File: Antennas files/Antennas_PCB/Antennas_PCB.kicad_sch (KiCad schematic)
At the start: 13 parts, among them U1 LMR14030SDDA, U2 TSR_1-2433

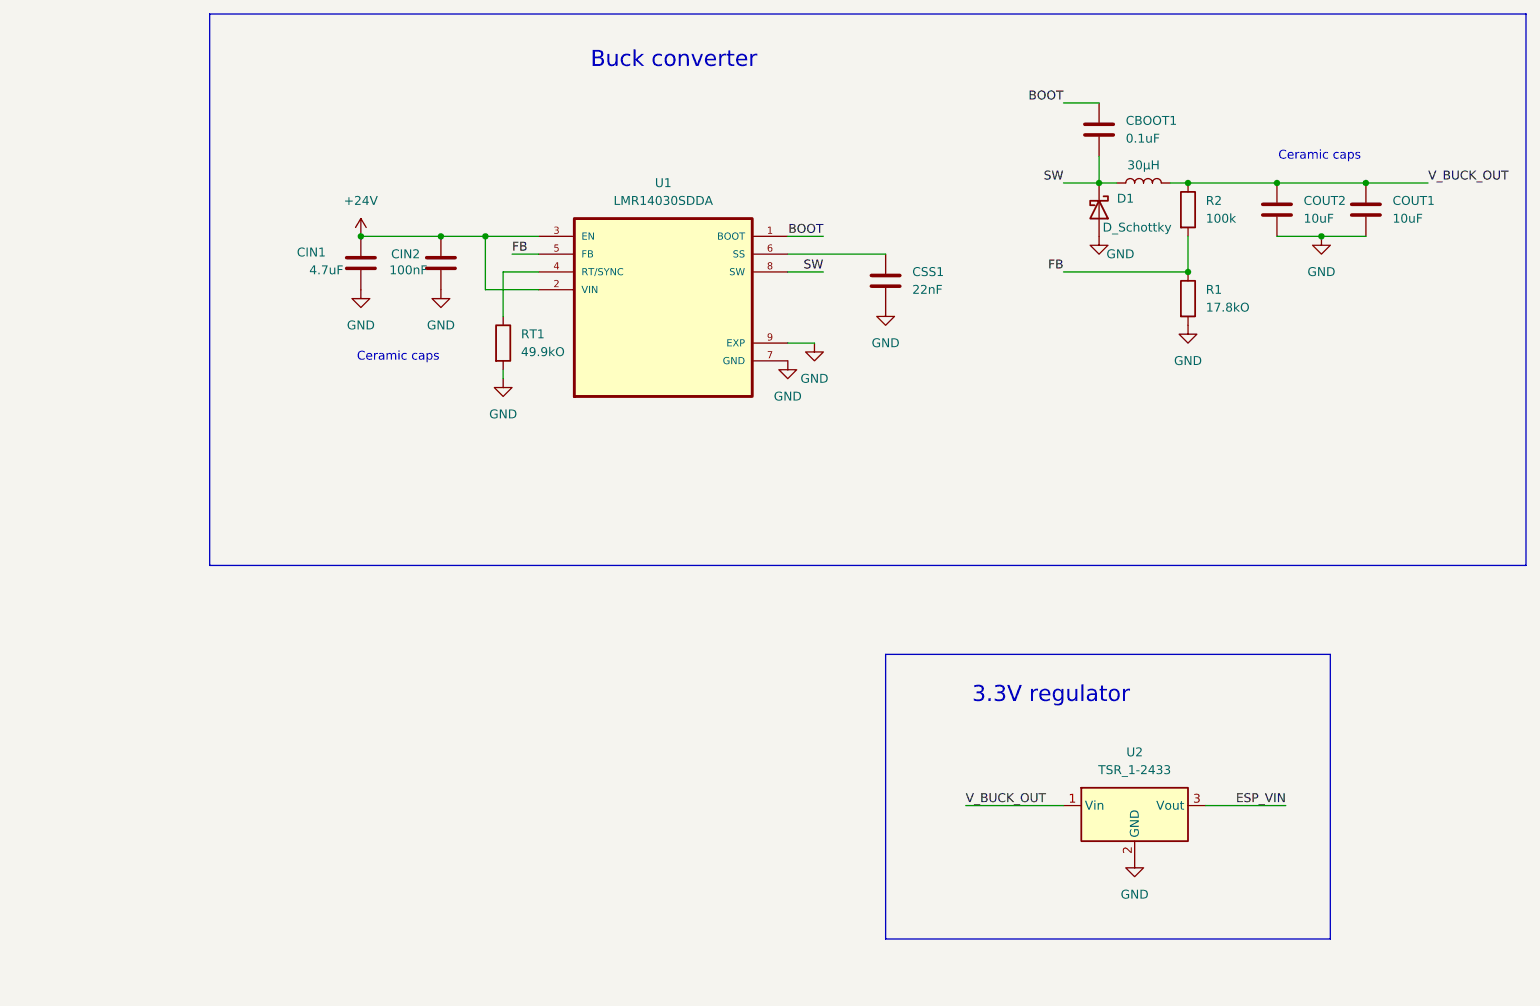
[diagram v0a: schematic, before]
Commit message: Add files via upload
pcb design for new buck and volt reg
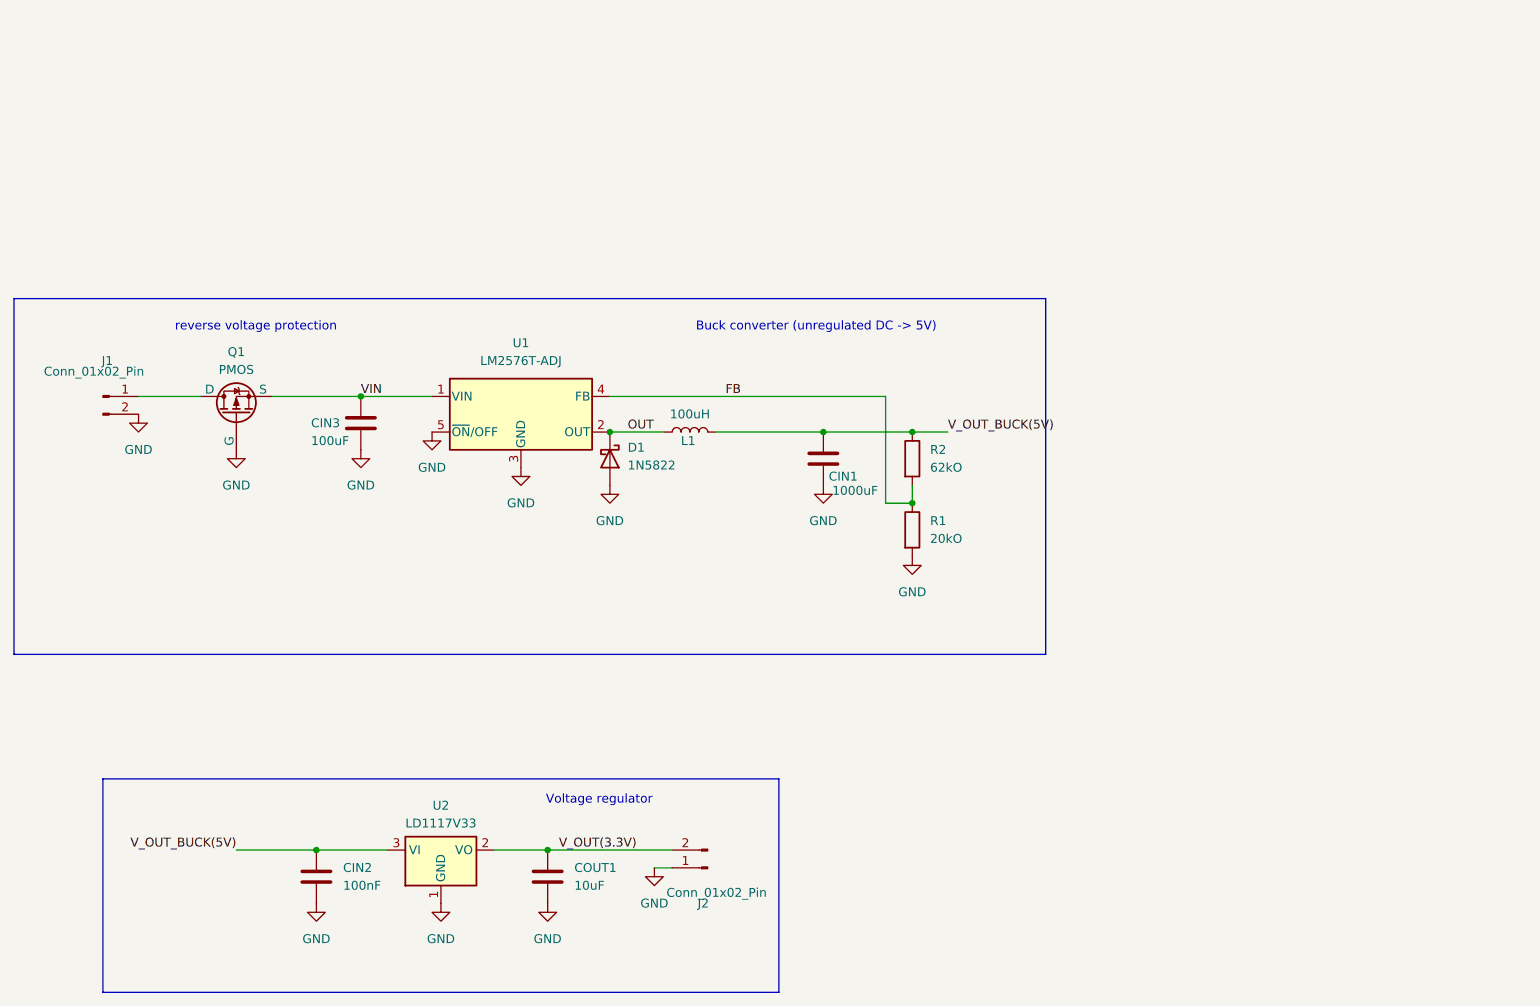
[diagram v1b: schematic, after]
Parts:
- removed CBOOT1: 0.1uF, Capacitor_SMD:C_0805_2012Metric_Pad1.18x1.45mm_HandSolder, symbol Device:C
- removed COUT2: 10uF, Capacitor_SMD:C_1206_3216Metric_Pad1.33x1.80mm_HandSolder, symbol Device:C
- removed CSS1: 22nF, Capacitor_SMD:C_0805_2012Metric_Pad1.18x1.45mm_HandSolder, symbol Device:C
- removed RT1: 49.9kO, Resistor_SMD:R_0805_2012Metric_Pad1.20x1.40mm_HandSolder, symbol Device:R
- removed U1: LMR14030SDDA, Package_SO:Texas_R-PDSO-G8_EP2.95x4.9mm_Mask2.4x3.1mm, symbol LMR14030SDDA:LMR14030SDDA
- removed U2: TSR_1-2433, Converter_DCDC:Converter_DCDC_TRACO_TSR-1_THT, symbol Converter_DCDC:TSR_1-2433
- added CIN3: 100uF, Capacitor_THT:C_Disc_D5.0mm_W2.5mm_P5.00mm, symbol Device:C
- added J1, J2: Conn_01x02_Pin, Connector_PinHeader_1.00mm:PinHeader_1x02_P1.00mm_Vertical, symbol Connector:Conn_01x02_Pin
- added Q1: PMOS, my_library:Untitled, symbol Simulation_SPICE:PMOS
- added U1: LM2576T-ADJ, Package_TO_SOT_THT:TO-220-5_Vertical, symbol Regulator_Switching:LM2576T-ADJ
- added U2: LD1117V33, Package_TO_SOT_THT:TO-220-3_Vertical, symbol Regulator_Linear:LD1117V33
- CIN1: value 4.7uF -> 1000uF; footprint Capacitor_SMD:C_0805_2012Metric_Pad1.18x1.45mm_HandSolder -> Capacitor_THT:C_Disc_D5.0mm_W2.5mm_P5.00mm
- CIN2: footprint Capacitor_SMD:C_0805_2012Metric_Pad1.18x1.45mm_HandSolder -> Capacitor_THT:C_Disc_D5.0mm_W2.5mm_P5.00mm
- COUT1: footprint Capacitor_SMD:C_1206_3216Metric_Pad1.33x1.80mm_HandSolder -> Capacitor_THT:C_Disc_D5.0mm_W2.5mm_P5.00mm
- D1: value D_Schottky -> 1N5822; footprint (none) -> Diode_THT:D_DO-201AD_P12.70mm_Horizontal
- L1: value 30µH -> 100uH; footprint (none) -> Inductor_THT:L_Axial_L6.6mm_D2.7mm_P10.16mm_Horizontal_Vishay_IM-2
- R1: value 17.8kO -> 20kO; footprint Resistor_SMD:R_0805_2012Metric_Pad1.20x1.40mm_HandSolder -> Resistor_THT:R_Axial_DIN0207_L6.3mm_D2.5mm_P10.16mm_Horizontal
- R2: value 100k -> 62kO; footprint Resistor_SMD:R_0805_2012Metric_Pad1.20x1.40mm_HandSolder -> Resistor_THT:R_Axial_DIN0207_L6.3mm_D2.5mm_P10.16mm_Horizontal
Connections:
- net FB: now also U1.4 (FB)
- net +24V renamed V_OUT_BUCK(5V)
- net V_OUT_BUCK(5V): now also L1.2, R2.1, U2.3 (VI)
- net EXP renamed GND
- net GND: now also CIN3.2, J1.2 (Pin_2), J2.1 (Pin_1), Q1.2 (G), U1.3 (GND), U1.5 (~{ON}/OFF), U2.1 (GND)
- net SW renamed OUT
- net OUT: now also U1.2 (OUT)
- removed net V_BUCK_OUT: COUT1.1, L1.2, R2.1
- new net: J1.1 (Pin_1), Q1.1 (D)
- new net VIN: CIN3.1, Q1.3 (S), U1.1 (VIN)
- new net V_OUT(3.3V): COUT1.1, J2.2 (Pin_2), U2.2 (VO)
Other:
- note added: "Buck converter (unregulated DC -> 5V)"
- note added: "Voltage regulator"
- note added: "reverse voltage protection"
- note removed: "3.3V regulator"
- note removed: "Buck converter"
- note removed: "Ceramic caps"
